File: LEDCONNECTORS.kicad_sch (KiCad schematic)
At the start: 6 parts, among them J901 FPC-0.5AL-12PB, J902 FPC-0.5AL-12PB, J903 FPC-0.5AL-12PB, J904 FPC-0.5AL-12PB, J905 FPC-0.5AL-12PB, J906 FPC-0.5AL-12PB

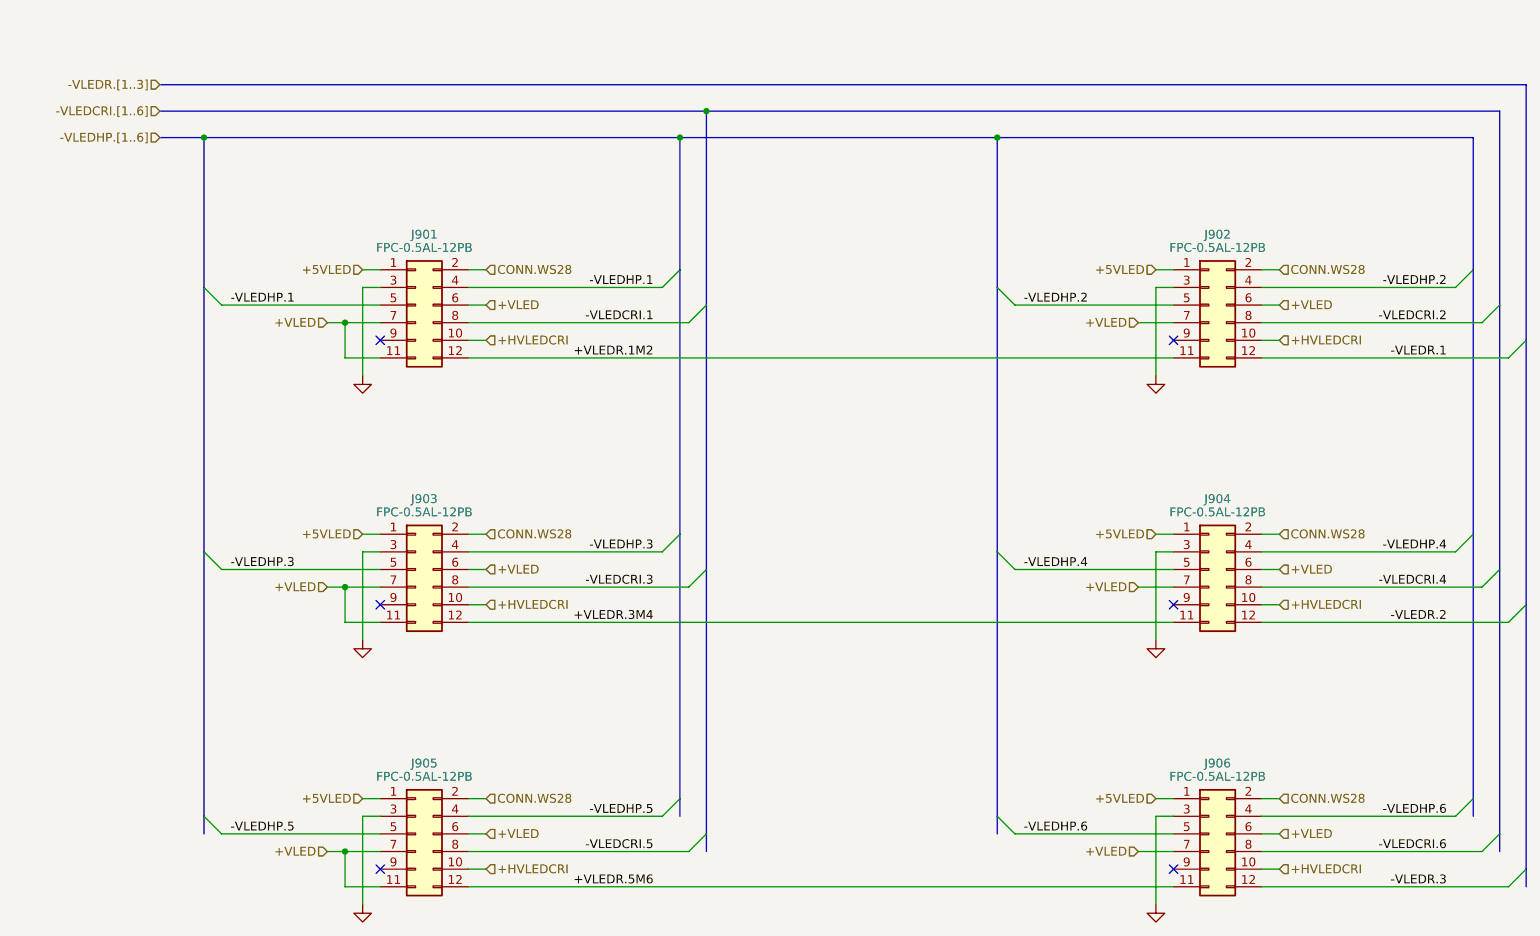
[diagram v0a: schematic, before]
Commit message: Add files via upload
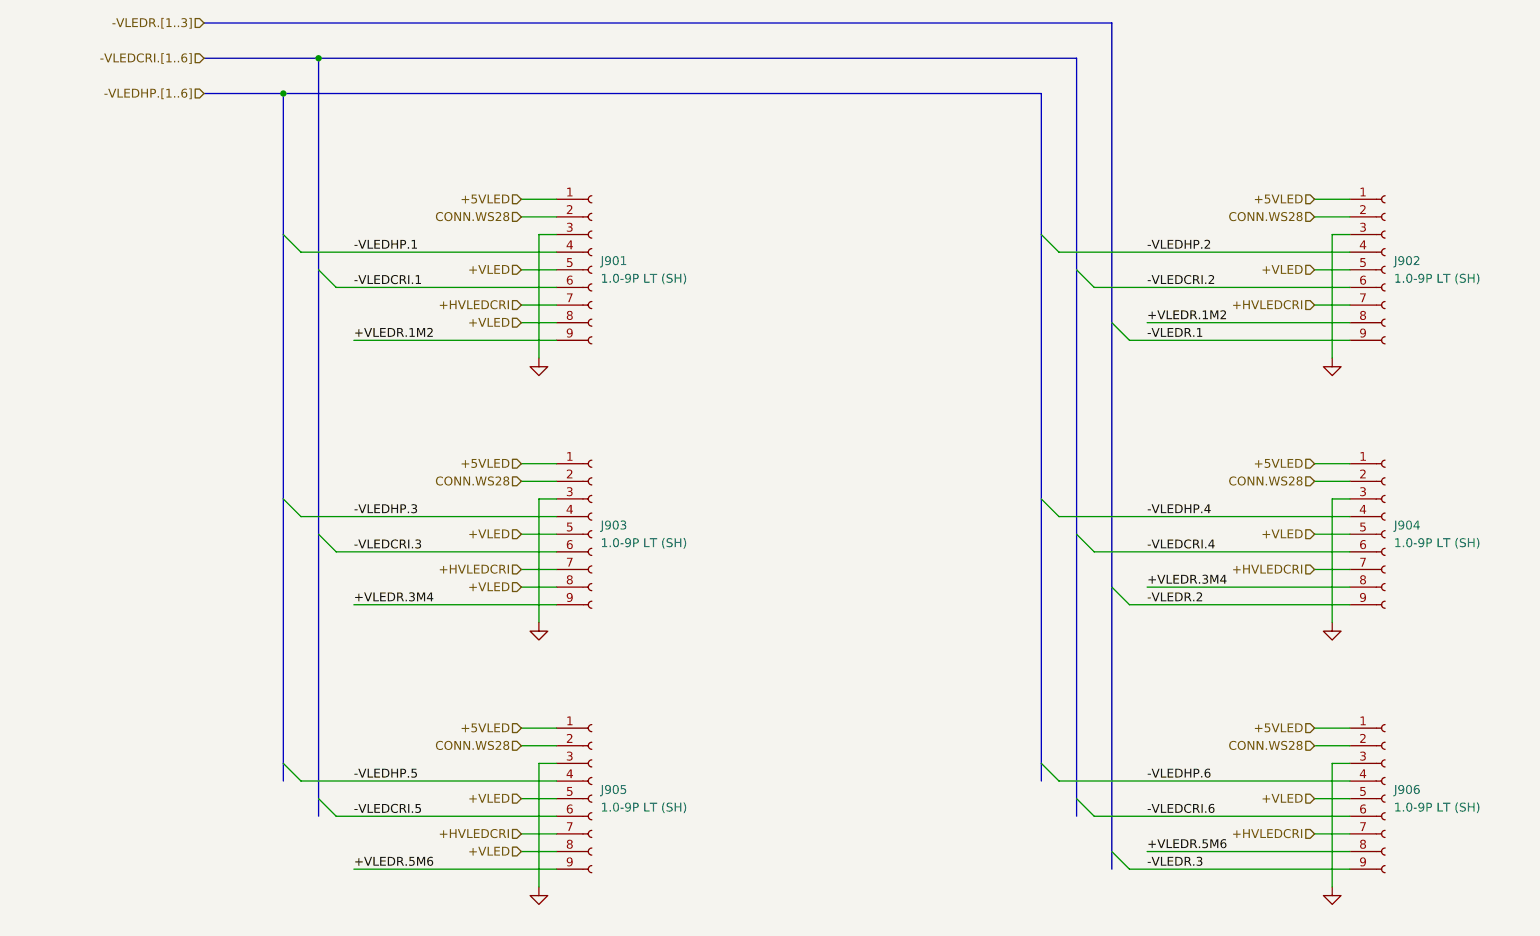
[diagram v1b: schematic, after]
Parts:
- removed J901, J902, J903, J904, J905, J906: FPC-0.5AL-12PB, Connectors FFC SMD:FPC-0.5AL-12PB, symbol Connector_Generic:Conn_02x06_Odd_Even
- added J901, J902, J903, J904, J905, J906: 1.0-9P LT (SH), Connectors SMD:1.0-9P LT (SH), symbol Connector:Conn_01x09_Socket
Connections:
- net +5VLED: now also J901.1 (Pin_1), J902.1 (Pin_1), J903.1 (Pin_1), J904.1 (Pin_1), J905.1 (Pin_1), J906.1 (Pin_1)
- net +HVLEDCRI: now also J901.7 (Pin_7), J902.7 (Pin_7), J903.7 (Pin_7), J904.7 (Pin_7), J905.7 (Pin_7), J906.7 (Pin_7)
- net +VLED: now also J901.5 (Pin_5), J901.8 (Pin_8), J902.5 (Pin_5), J903.5 (Pin_5), J903.8 (Pin_8), J904.5 (Pin_5), J905.5 (Pin_5), J905.8 (Pin_8), J906.5 (Pin_5)
- net +VLEDR.1M2: now also J901.9 (Pin_9), J902.8 (Pin_8)
- net +VLEDR.3M4: now also J903.9 (Pin_9), J904.8 (Pin_8)
- net +VLEDR.5M6: now also J905.9 (Pin_9), J906.8 (Pin_8)
- net -VLEDCRI.1: now also J901.6 (Pin_6)
- net -VLEDCRI.2: now also J902.6 (Pin_6)
- net -VLEDCRI.3: now also J903.6 (Pin_6)
- net -VLEDCRI.4: now also J904.6 (Pin_6)
- net -VLEDCRI.5: now also J905.6 (Pin_6)
- net -VLEDCRI.6: now also J906.6 (Pin_6)
- net -VLEDHP.1: now also J901.4 (Pin_4)
- net -VLEDHP.2: now also J902.4 (Pin_4)
- net -VLEDHP.3: now also J903.4 (Pin_4)
- net -VLEDHP.4: now also J904.4 (Pin_4)
- net -VLEDHP.5: now also J905.4 (Pin_4)
- net -VLEDHP.6: now also J906.4 (Pin_4)
- net -VLEDR.1: now also J902.9 (Pin_9)
- net -VLEDR.2: now also J904.9 (Pin_9)
- net -VLEDR.3: now also J906.9 (Pin_9)
- net CONN.WS28: now also J901.2 (Pin_2), J902.2 (Pin_2), J903.2 (Pin_2), J904.2 (Pin_2), J905.2 (Pin_2), J906.2 (Pin_2)
- net GND: now also J901.3 (Pin_3), J902.3 (Pin_3), J903.3 (Pin_3), J904.3 (Pin_3), J905.3 (Pin_3), J906.3 (Pin_3)
- no-connect marks 6 -> 0
